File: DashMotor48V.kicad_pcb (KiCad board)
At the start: 4 copper layers, 71.8 x 70.7 mm, 79 parts, among them CN3(OUT)1 XT30(2+2)PB-M.G.B, CN3(OUT)2 XT30(2+2)PB-M.G.B, J1 BM07B-SRSS-TB, J2 BM07B-SRSS-TB, Q1 FDMS039N08B, Q2 FDMS039N08B, Q3 FDMS039N08B, Q4 FDMS039N08B, Q5 FDMS039N08B, Q6 FDMS039N08B, U1 TPS629203DRLR, U2 TPS629203DRLR, U3 DRV8353SRTAR, U4 STM32F446RCT6, U5 MA732GQ-Z, U6 MCP2542FD-E/MF, Y1 CSTNE8M00G550000R0

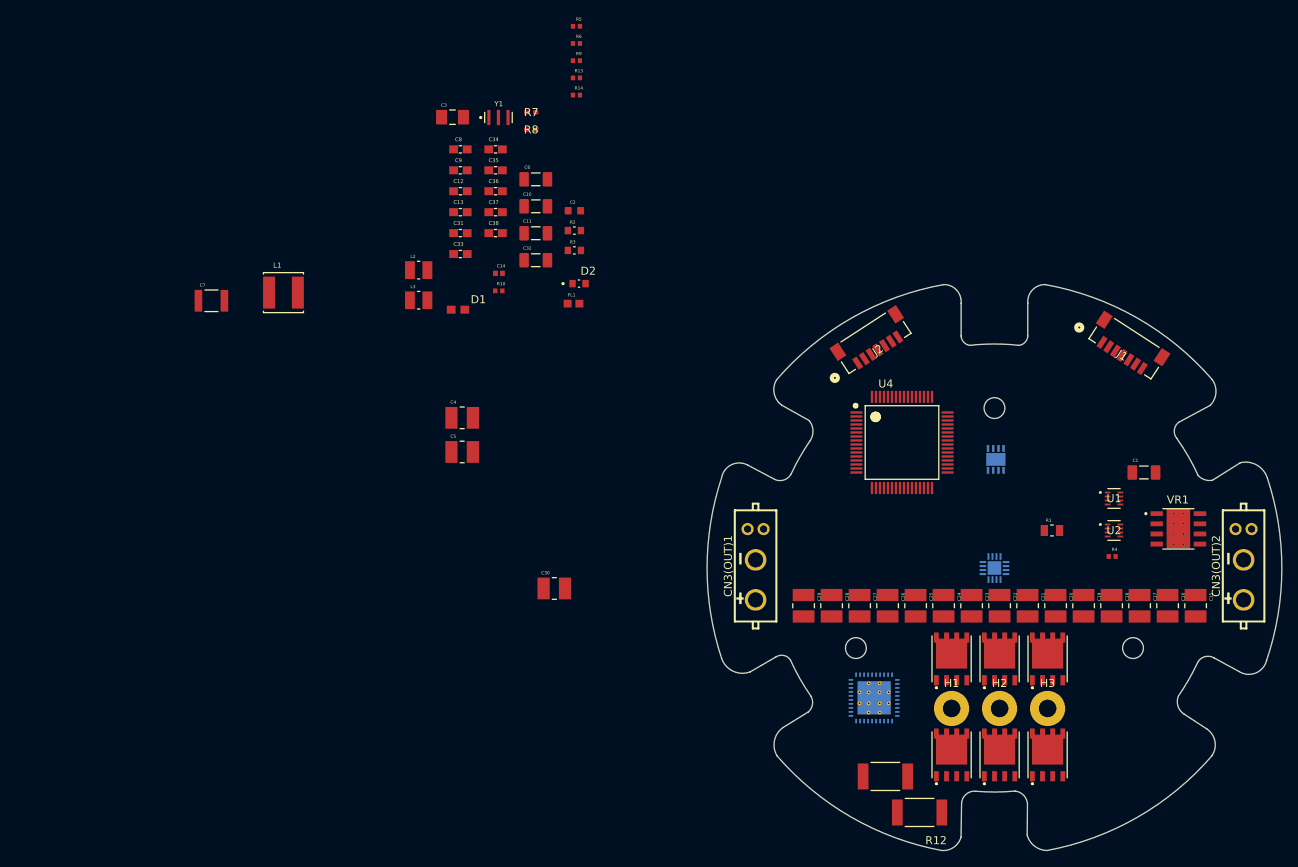
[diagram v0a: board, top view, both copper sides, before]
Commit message: put onto the board
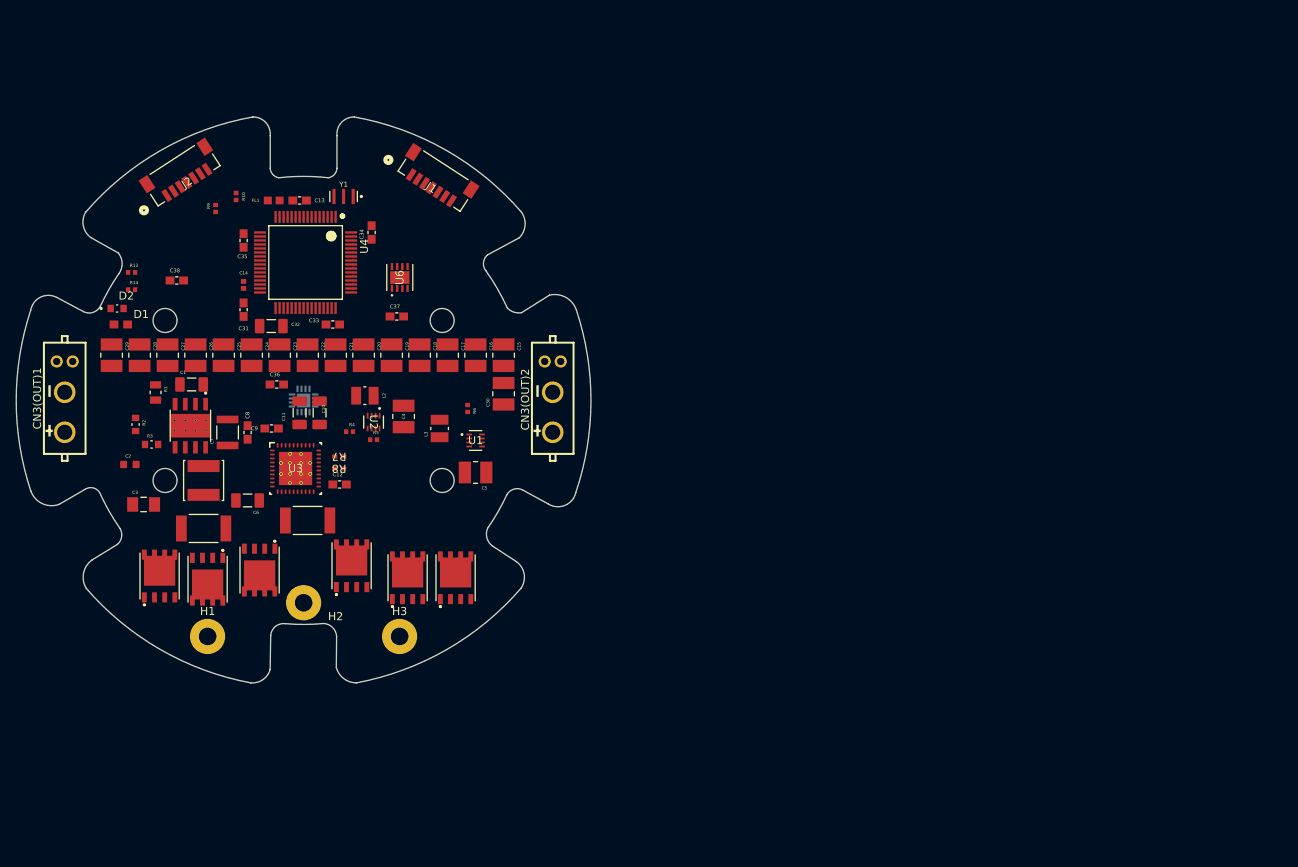
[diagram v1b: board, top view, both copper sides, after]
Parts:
- U3, U6: moved to F.Cu
- moved VR1 124.2 mm to (85.8, 103.2), turned to -90 degrees
- moved C1 119.5 mm to (86.0, 98.0)
- moved R1 113.4 mm to (81.5, 99.0), turned to -90 degrees
- moved Q1 99.5 mm to (82.0, 122.1)
- moved R4 96.6 mm to (105.7, 103.9)
- moved Q2 95.6 mm to (88.0, 122.1), turned to 180 degrees
- moved Q4 95.4 mm to (94.5, 121.0), turned to 180 degrees
- moved U2 93.5 mm to (108.7, 102.7), turned to -90 degrees
- moved H1 93.4 mm to (88.0, 129.5)
- moved C15 92.0 mm to (125.0, 94.3)
- moved C16 92.0 mm to (121.5, 94.3)
- moved C17 92.0 mm to (118.0, 94.3)
- moved C18 92.0 mm to (114.5, 94.3)
- moved C19 92.0 mm to (111.0, 94.3)
- moved C20 92.0 mm to (107.5, 94.3)
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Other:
- outline, holes or cut-outs redrawn
